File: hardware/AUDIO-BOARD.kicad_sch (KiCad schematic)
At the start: 5 parts, among them J1 CON_USB_GCT_USB4105_REVA, J5 SD-CARD-MEM2051-00-195-00-A, M1 MNT, M2 MNT, M3 MNT

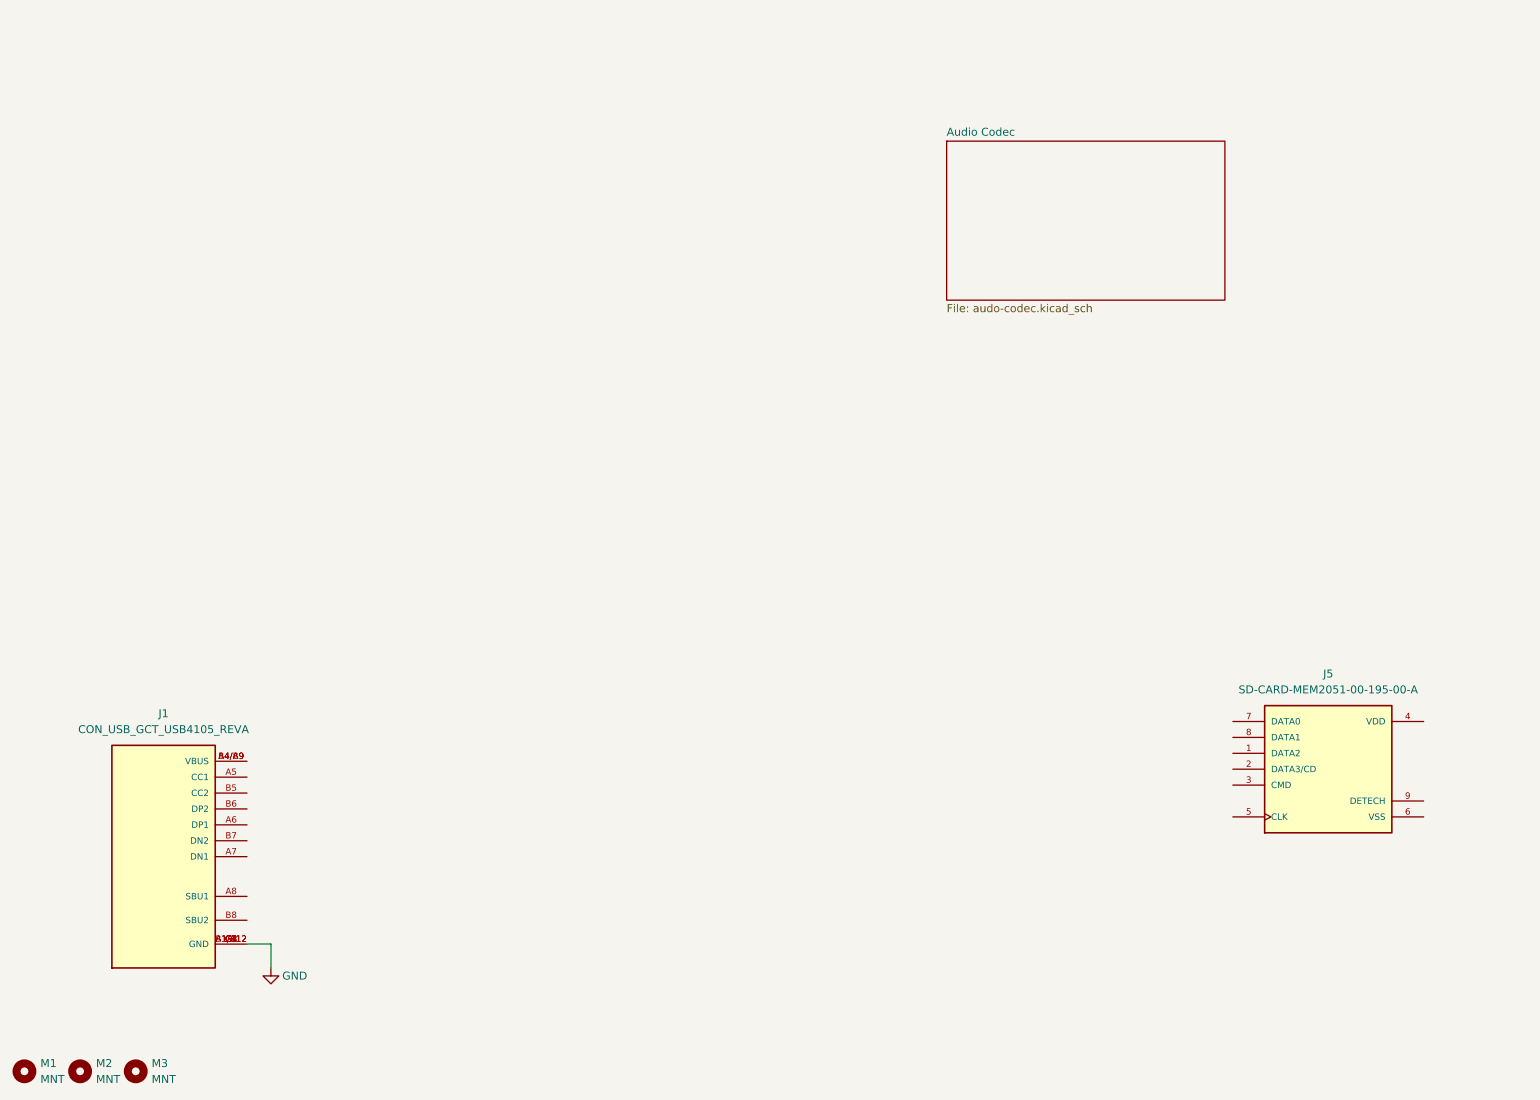
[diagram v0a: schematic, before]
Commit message: Project setup
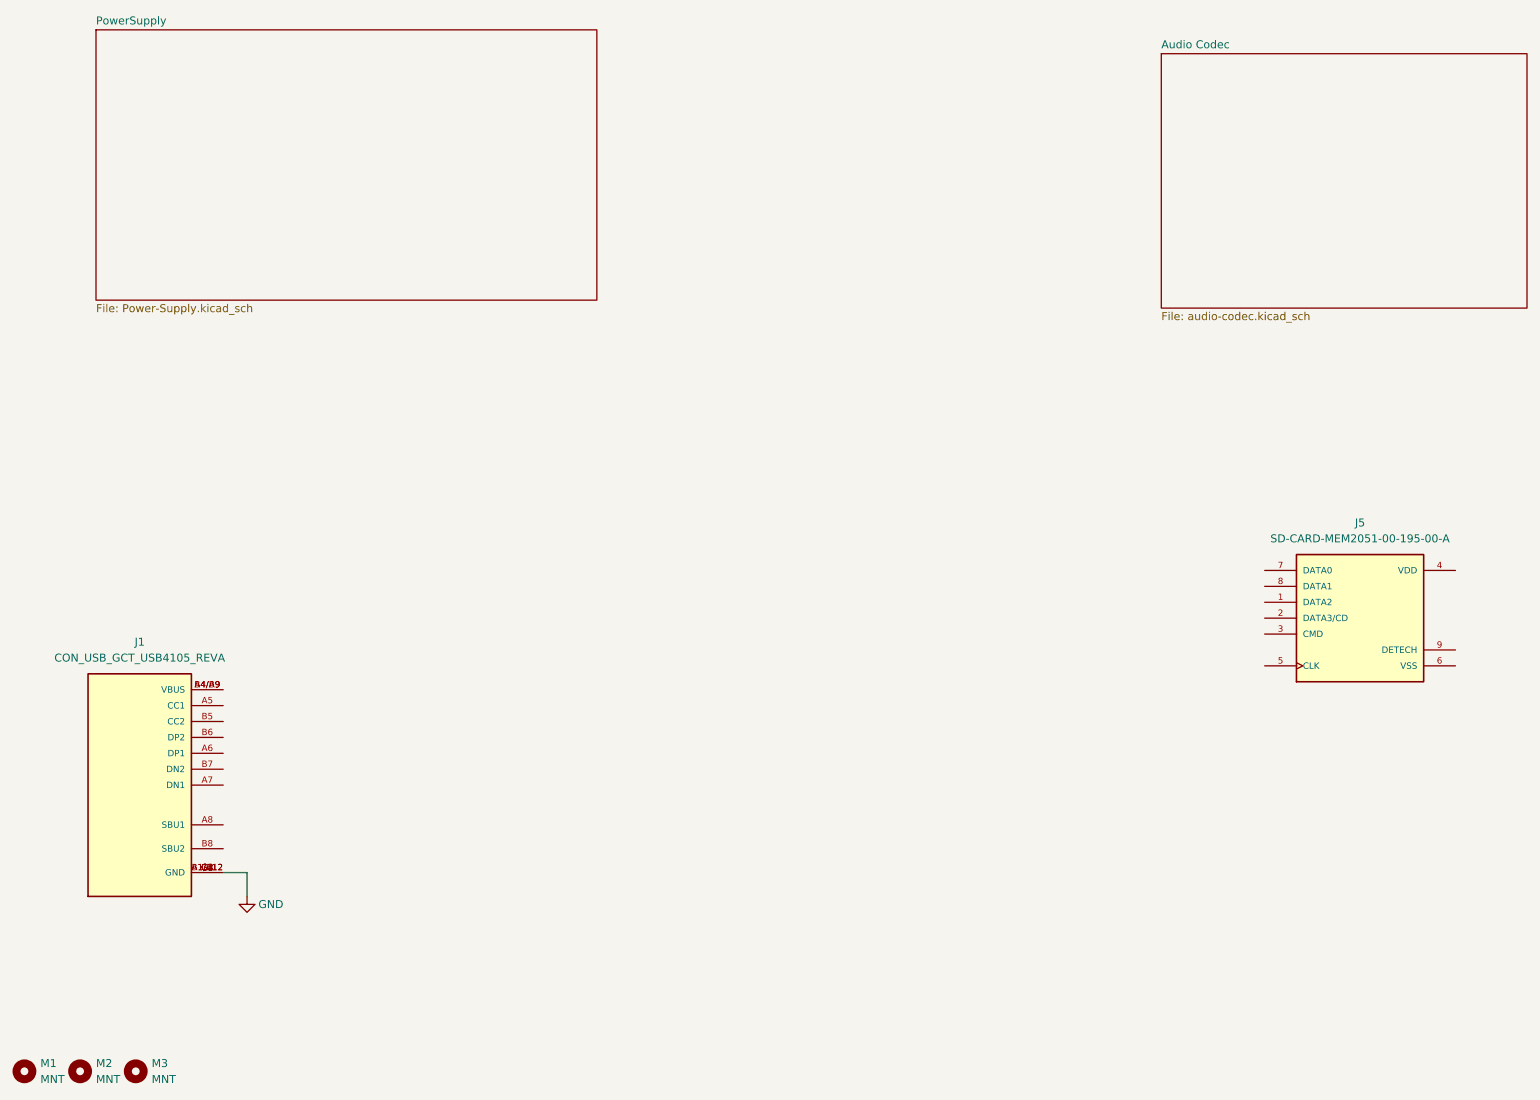
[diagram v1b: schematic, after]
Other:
- added sheet PowerSupply (Power-Supply.kicad_sch)
- sheet Audio Codec: file audo-codec.kicad_sch -> audio-codec.kicad_sch
- moved on the sheet: J1, J5
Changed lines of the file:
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@@
 (kicad_sch (version 20211123) (generator eeschema)
   (paper "A4")
-  (wire (pts (xy 55.88 171.45) (xy 52.07 171.45))
+  (wire (pts (xy 52.07 160.02) (xy 48.26 160.02))
     (stroke (width 0) (type default) (color 0 0 0 0))
   )
-  (wire (pts (xy 55.88 175.26) (xy 55.88 171.45))
+  (wire (pts (xy 52.07 163.83) (xy 52.07 160.02))
     (stroke (width 0) (type default) (color 0 0 0 0))
   )
   (symbol (lib_id "Mechanical:MountingHole") (at 34.29 191.77 0) (unit 1)
-    (in_bom yes) (on_board yes) (fields_autoplaced)
+    (in_bom yes) (on_board yes)
     (property "Reference" "M3" (id 0) (at 36.83 190.4999 0)
       (effects (font (size 1.27 1.27)) (justify left))
@@
     )
   )
-  (symbol (lib_id "1KiCadLib:CON_USB_GCT_USB4105_REVA") (at 31.75 152.4 0) (unit 1)
+  (symbol (lib_id "1KiCadLib:CON_USB_GCT_USB4105_REVA") (at 27.94 140.97 0) (unit 1)
     (in_bom yes) (on_board yes) (fields_autoplaced)
-    (property "Reference" "J1" (id 0) (at 38.735 134.62 0))
-    (property "Value" "CON_USB_GCT_USB4105_REVA" (id 1) (at 38.735 137.16 0))
-    (property "Footprint" "1KiCadLib:CON_USB_GCT_USB4105_REVA" (id 2) (at 12.7 137.16 0)
+    (property "Reference" "J1" (id 0) (at 34.925 123.19 0))
+    (property "Value" "CON_USB_GCT_USB4105_REVA" (id 1) (at 34.925 125.73 0))
+    (property "Footprint" "1KiCadLib:CON_USB_GCT_USB4105_REVA" (id 2) (at 8.89 125.73 0)
       (effects (font (size 1.27 1.27)) (justify left bottom) hide)
     )
-    (property "Datasheet" "" (id 3) (at 31.75 152.4 0)
+    (property "Datasheet" "" (id 3) (at 27.94 140.97 0)
       (effects (font (size 1.27 1.27)) (justify left bottom) hide)
     )
-    (property "MAXIMUM_PACKAGE_HEIGHT" "3.31 mm" (id 4) (at 25.4 146.05 0)
+    (property "MAXIMUM_PACKAGE_HEIGHT" "3.31 mm" (id 4) (at 21.59 134.62 0)
       (effects (font (size 1.27 1.27)) (justify left bottom) hide)
     )
-    (property "MANUFACTURER" "GCT" (id 5) (at 31.75 152.4 0)
+    (property "MANUFACTURER" "GCT" (id 5) (at 27.94 140.97 0)
       (effects (font (size 1.27 1.27)) (justify left bottom) hide)
     )
-    (property "PARTREV" "0.2" (id 6) (at 31.75 152.4 0)
+    (property "PARTREV" "0.2" (id 6) (at 27.94 140.97 0)
       (effects (font (size 1.27 1.27)) (justify left bottom) hide)
     )
-    (property "STANDARD" "Manufacturer Recommendations" (id 7) (at 13.97 134.62 0)
+    (property "STANDARD" "Manufacturer Recommendations" (id 7) (at 10.16 123.19 0)
       (effects (font (size 1.27 1.27)) (justify left bottom) hide)
     )
@@
     (pin "G4")
   )
-  (symbol (lib_id "power:GND") (at 55.88 175.26 0) (unit 1)
+  (symbol (lib_id "power:GND") (at 52.07 163.83 0) (unit 1)
     (in_bom yes) (on_board yes)
-    (property "Reference" "#PWR0103" (id 0) (at 55.88 181.61 0)
+    (property "Reference" "#PWR0103" (id 0) (at 52.07 170.18 0)
       (effects (font (size 1.27 1.27)) hide)
     )
-    (property "Value" "GND" (id 1) (at 59.69 176.53 0))
-    (property "Footprint" "" (id 2) (at 55.88 175.26 0)
+    (property "Value" "GND" (id 1) (at 55.88 165.1 0))
+    (property "Footprint" "" (id 2) (at 52.07 163.83 0)
       (effects (font (size 1.27 1.27)) hide)
     )
-    (property "Datasheet" "" (id 3) (at 55.88 175.26 0)
+    (property "Datasheet" "" (id 3) (at 52.07 163.83 0)
       (effects (font (size 1.27 1.27)) hide)
     )
@@
   )
   (symbol (lib_id "Mechanical:MountingHole") (at 25.4 191.77 0) (unit 1)
-    (in_bom yes) (on_board yes) (fields_autoplaced)
+    (in_bom yes) (on_board yes)
     (property "Reference" "M2" (id 0) (at 27.94 190.4999 0)
       (effects (font (size 1.27 1.27)) (justify left))
@@
     )
   )
-  (symbol (lib_id "1KiCadLib:SD-CARD-MEM2051-00-195-00-A") (at 224.79 143.51 0) (unit 1)
+  (symbol (lib_id "1KiCadLib:SD-CARD-MEM2051-00-195-00-A") (at 229.87 119.38 0) (unit 1)
     (in_bom yes) (on_board yes) (fields_autoplaced)
-    (property "Reference" "J5" (id 0) (at 224.79 128.27 0))
-    (property "Value" "SD-CARD-MEM2051-00-195-00-A" (id 1) (at 224.79 130.81 0))
-    (property "Footprint" "1KiCadLib:SD-CARD-MEM2051-00-195-00-A" (id 2) (at 222.25 128.27 0)
+    (property "Reference" "J5" (id 0) (at 229.87 104.14 0))
+    (property "Value" "SD-CARD-MEM2051-00-195-00-A" (id 1) (at 229.87 106.68 0))
+    (property "Footprint" "1KiCadLib:SD-CARD-MEM2051-00-195-00-A" (id 2) (at 227.33 104.14 0)
       (effects (font (size 1.27 1.27)) (justify bottom) hide)
     )
-    (property "Datasheet" "https://www.mouser.fr/ProductDetail/GCT/MEM2051-00-195-00-A?qs=KUoIvG%2F9Ilat7yfJRNWXUQ%3D%3D" (id 3) (at 224.79 129.54 0)
+    (property "Datasheet" "https://www.mouser.fr/ProductDetail/GCT/MEM2051-00-195-00-A?qs=KUoIvG%2F9Ilat7yfJRNWXUQ%3D%3D" (id 3) (at 229.87 105.41 0)
       (effects (font (size 1.27 1.27)) hide)
     )
-    (property "Manufacturer" "GCT" (id 4) (at 224.79 143.51 0)
+    (property "Manufacturer" "GCT" (id 4) (at 229.87 119.38 0)
       (effects (font (size 1.27 1.27)) (justify bottom) hide)
     )
-    (property "MPN" "MEM2051-00-195-00-A" (id 5) (at 220.98 121.92 0)
+    (property "MPN" "MEM2051-00-195-00-A" (id 5) (at 226.06 97.79 0)
       (effects (font (size 1.27 1.27)) hide)
     )
-    (property "Mouser" "640-MEM20510019500A" (id 6) (at 219.71 124.46 0)
+    (property "Mouser" "640-MEM20510019500A" (id 6) (at 224.79 100.33 0)
       (effects (font (size 1.27 1.27)) hide)
     )
@@
     (pin "9")
   )
-  (sheet (at 163.83 43.18) (size 44.45 25.4) (fields_autoplaced)
+  (sheet (at 198.12 29.21) (size 58.42 40.64) (fields_autoplaced)
     (stroke (width 0.1524) (type solid) (color 128 77 0 1))
     (fill (color 255 255 194 1.0000))
-    (property "Sheet name" "Audio Codec" (id 0) (at 163.83 42.4684 0)
+    (property "Sheet name" "Audio Codec" (id 0) (at 198.12 28.4984 0)
       (effects (font (size 1.27 1.27)) (justify left bottom))
     )
-    (property "Sheet file" "audo-codec.kicad_sch" (id 1) (at 163.83 69.1646 0)
+    (property "Sheet file" "audio-codec.kicad_sch" (id 1) (at 198.12 70.4346 0)
+      (effects (font (size 1.27 1.27)) (justify left top))
+    )
+  )
+  (sheet (at 27.94 25.4) (size 80.01 43.18) (fields_autoplaced)
+    (stroke (width 0.1524) (type solid) (color 0 0 0 0))
+    (fill (color 0 0 0 0.0000))
+    (property "Sheet name" "PowerSupply" (id 0) (at 27.94 24.6884 0)
+      (effects (font (size 1.27 1.27)) (justify left bottom))
+    )
+    (property "Sheet file" "Power-Supply.kicad_sch" (id 1) (at 27.94 69.1646 0)
       (effects (font (size 1.27 1.27)) (justify left top))
     )
@@
     (path "/" (page "1"))
     (path "/5942f19b-9c4c-4b0c-8e9c-1608ad5e1222" (page "2"))
+    (path "/a72be1e0-9af1-4c8b-a80a-e23a2ce6ded3" (page "3"))
   )
   (symbol_instances
